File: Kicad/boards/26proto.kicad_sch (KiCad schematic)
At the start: 4 parts, among them J1 5051104096, U1 MOUDLE-SEEEDUINO-XIAO-ESP32C3, U2 MOUDLE-SEEEDUINO-XIAO-ESP32C3, U3 MAX3485

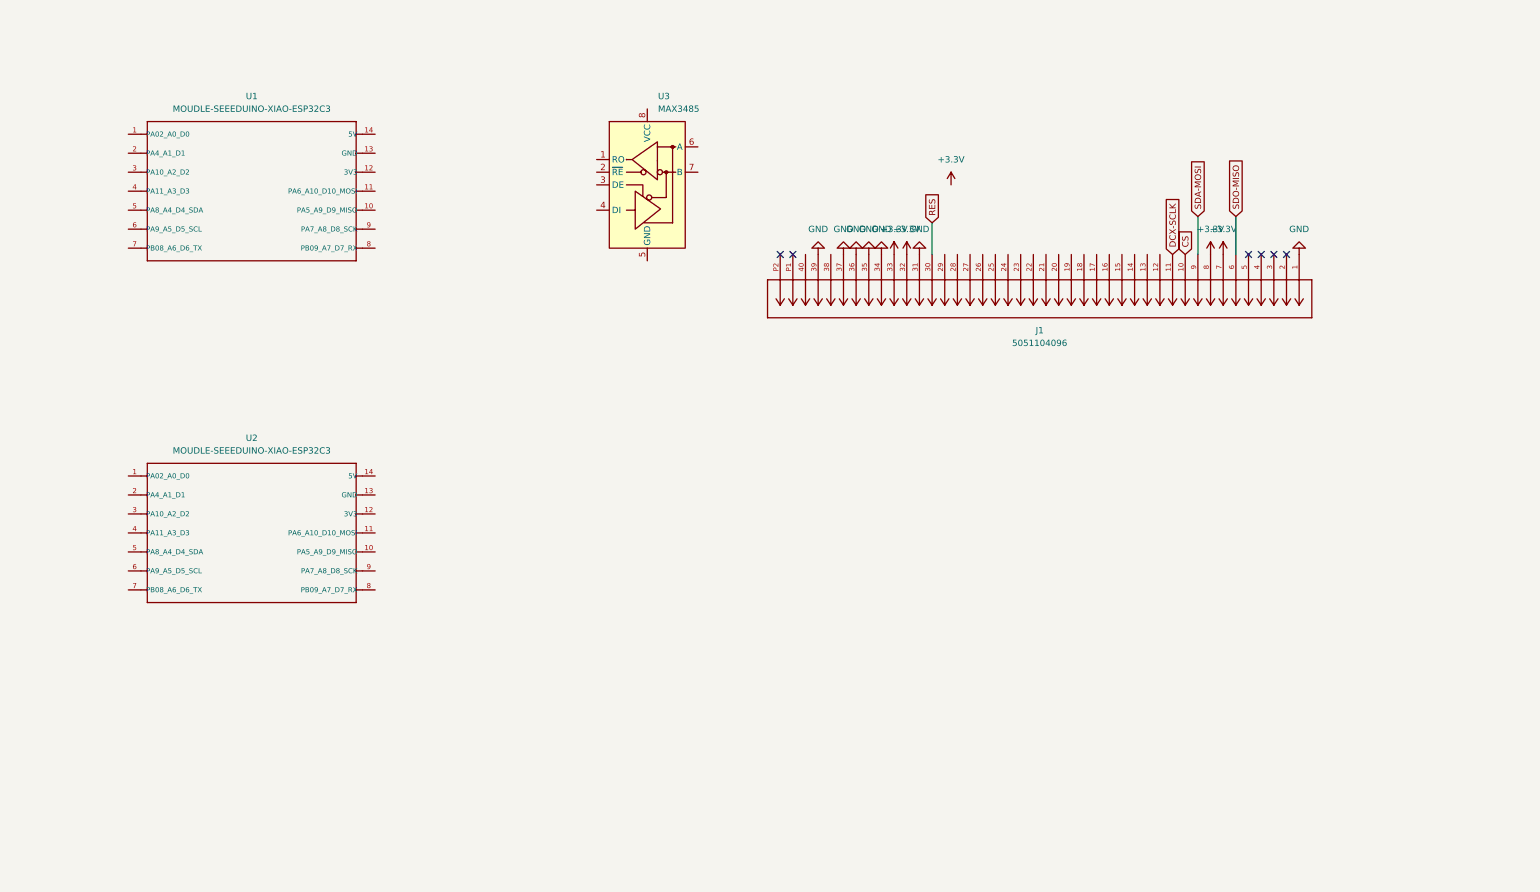
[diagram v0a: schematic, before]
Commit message: edited sch
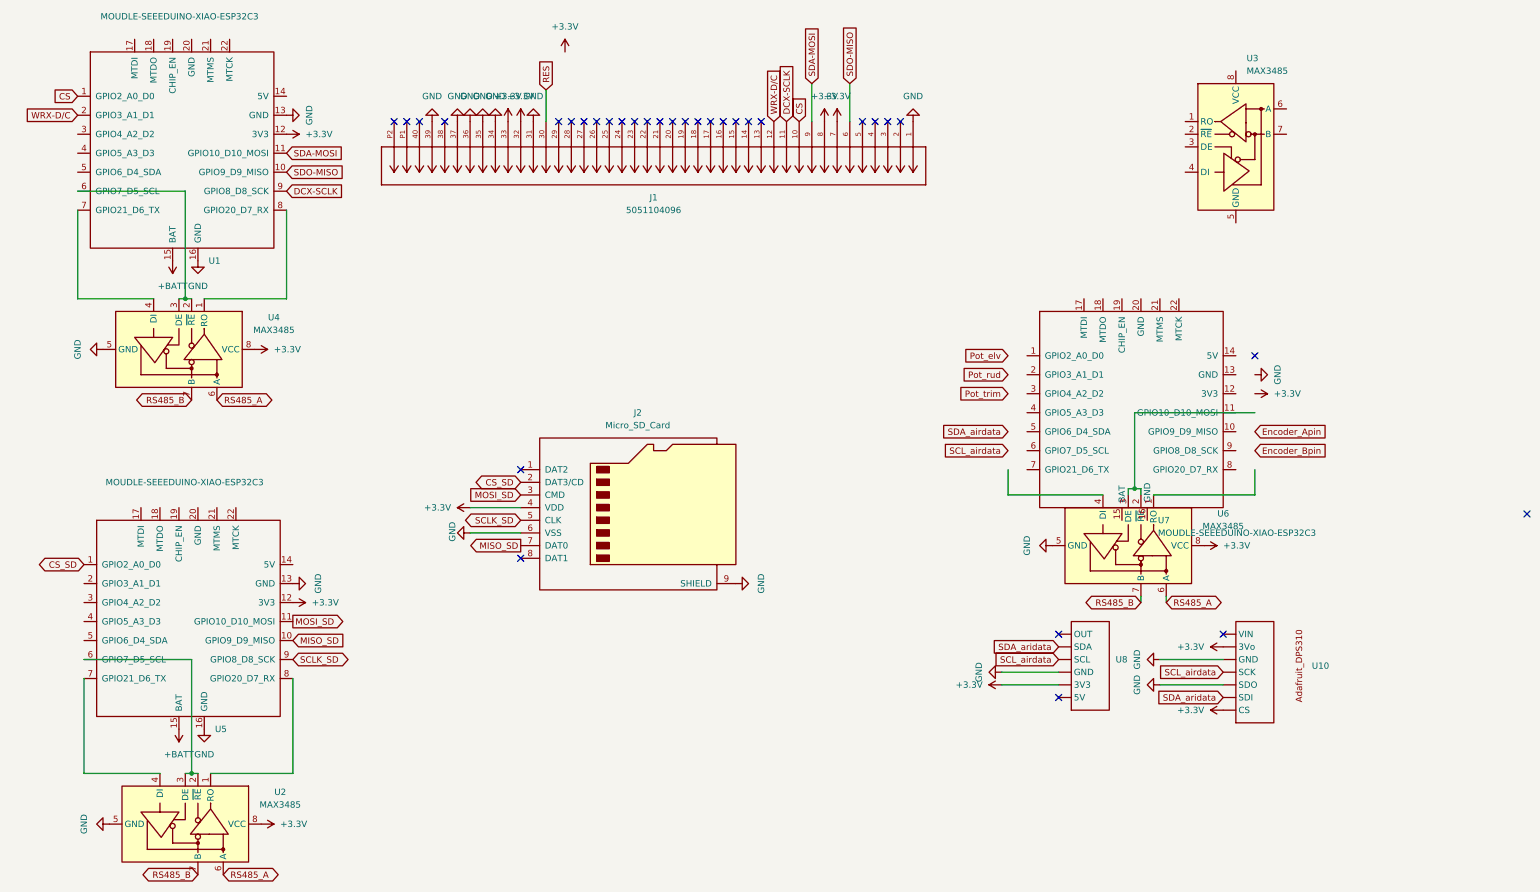
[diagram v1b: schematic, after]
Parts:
- removed U2: MOUDLE-SEEEDUINO-XIAO-ESP32C3, MOUDLE14P-SMD-2.54-21X17.8MM, symbol XIAO_ESP32C3:MOUDLE-SEEEDUINO-XIAO-ESP32C3
- added J2: Micro_SD_Card, symbol Connector:Micro_SD_Card
- added U10: ~, symbol New_Library:Adafruit_DPS310
- added U2, U4, U6: MAX3485, Package_SO:SOIC-8_3.9x4.9mm_P1.27mm, symbol Interface_UART:MAX3485
- added U5, U7: MOUDLE-SEEEDUINO-XIAO-ESP32C3, MOUDLE14P-SMD-2.54-21X17.8MM, symbol Seeed_Studio_XIAO_Series:XIAO-ESP32-C3-SMD
- added U8: ~, symbol New_Library:AS5600
- U1: symbol XIAO_ESP32C3:MOUDLE-SEEEDUINO-XIAO-ESP32C3 -> Seeed_Studio_XIAO_Series:XIAO-ESP32-C3-SMD
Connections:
- net +3.3V: now also U1.12 (3V3), J2.4 (VDD), U10. (VIN), U2.8 (VCC), U4.8 (VCC), U5.12 (3V3), U6.8 (VCC), U8. (OUT)
- net CS: now also U1.1 (GPIO2_A0_D0)
- net DCX-SCLK: now also U1.9 (GPIO8_D8_SCK)
- net GND: now also U1.13 (GND), U1.16 (GND), J2.6 (VSS), J2.9 (SHIELD), U10. (VIN), U2.5 (GND), U4.5 (GND), U5.13 (GND), U5.16 (GND), U6.5 (GND), U8. (OUT)
- net SDA-MOSI: now also U1.11 (GPIO10_D10_MOSI)
- net SDO-MISO: now also U1.10 (GPIO9_D9_MISO)
- net WRX-D/C: now reaches J1.12
- net WRX-D/C: now also U1.2 (GPIO3_A1_D1)
- net at U1.6 (GPIO7_D5_SCL): now also U4.2 (~{RE}), U4.3 (DE)
- net at U1.7 (GPIO21_D6_TX): now also U4.4 (DI)
- net at U1.8 (GPIO20_D7_RX): now also U4.1 (RO)
- new net: U2.1 (RO), U5.8 (GPIO20_D7_RX)
- new net: U2.2 (~{RE}), U2.3 (DE), U5.6 (GPIO7_D5_SCL)
- new net: U2.4 (DI), U5.7 (GPIO21_D6_TX)
- new net: U6.2 (~{RE}), U6.3 (DE)
- new net +BATT: U1.15 (BAT), U5.15 (BAT)
- new net CS_SD: J2.2 (DAT3/CD), U5.1 (GPIO2_A0_D0)
- new net MISO_SD: J2.7 (DAT0), U5.10 (GPIO9_D9_MISO)
- new net MOSI_SD: J2.3 (CMD), U5.11 (GPIO10_D10_MOSI)
- new net RS485_A: U2.6 (A), U4.6 (A), U6.6 (A)
- new net RS485_B: U2.7 (B), U4.7 (B), U6.7 (B)
- new net SCLK_SD: J2.5 (CLK), U5.9 (GPIO8_D8_SCK)
- new net SCL_airdata: U10. (VIN), U8. (OUT)
- new net SDA_aridata: U10. (VIN), U8. (OUT)
- no-connect marks 6 -> 32
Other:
- moved on the sheet: J1, U1, U3
